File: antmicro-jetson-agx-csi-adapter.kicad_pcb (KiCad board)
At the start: 4 copper layers, 73.6 x 41 mm, 102 parts, among them IC1 MAX1708EEE+, J1 QTH-060-03-L-D-A, J2 WE_68715014522_ONE-SIDE, J3 WE_68715014022, J4 SM04B-SRSS-TB-LF-SN, J5 SM06B-SRSS-TB(LF)(SN), J6 SM09B-SRSS-TB(LF)(SN), Q1 BSS138AKA, U1 PCA9547BS,118, U2 NTS0102DP

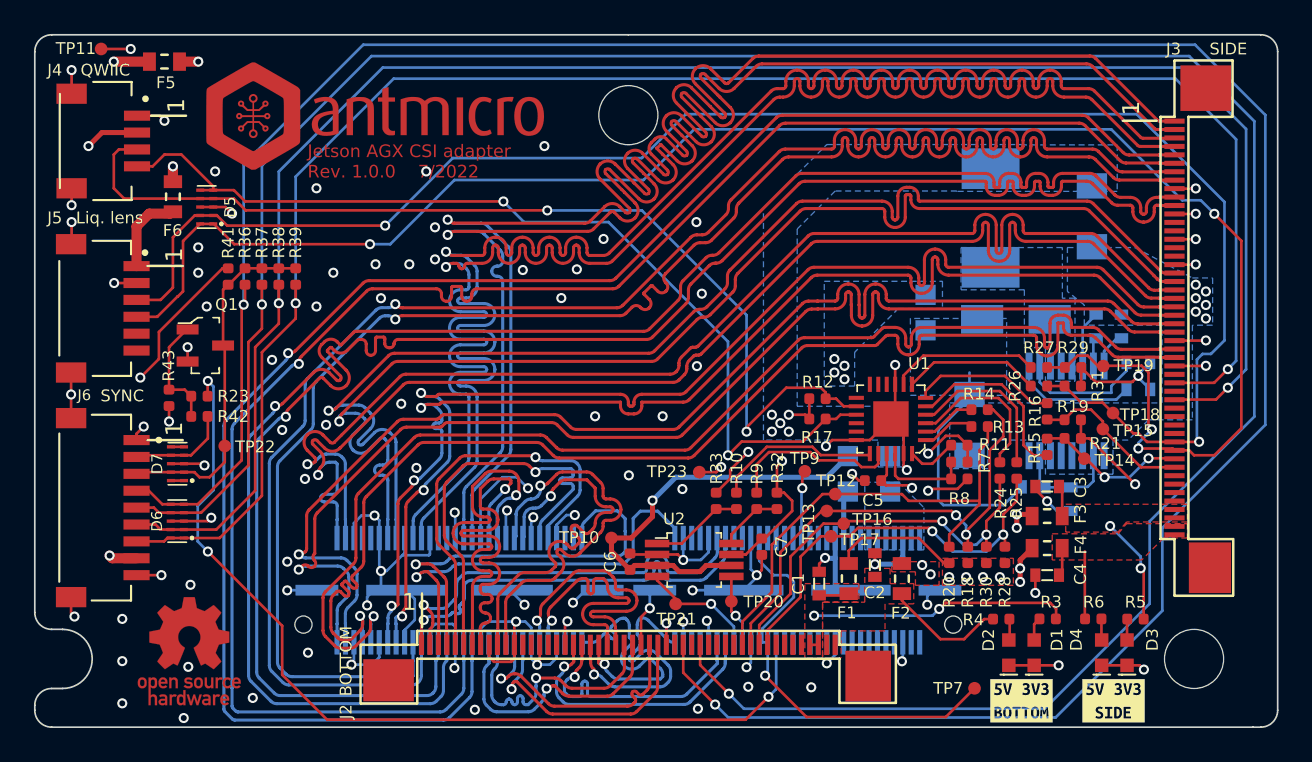
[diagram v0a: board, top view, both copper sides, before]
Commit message: [#60956] WiP Update symbols references
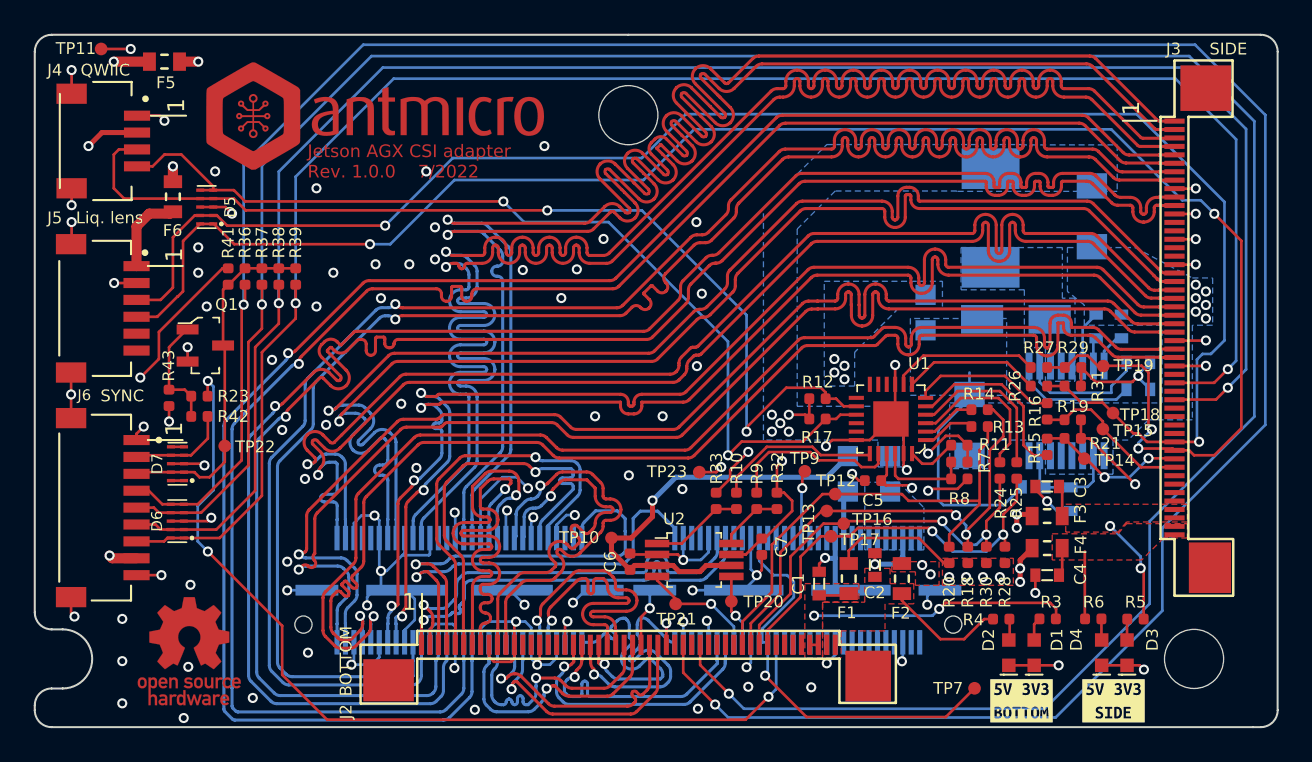
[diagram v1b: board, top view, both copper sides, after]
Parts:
- C1, C10, C11, C2, C3, C4, C9: footprint antmicro-jetson-agx-csi-adapter-footprints:0603-cap -> antmicro-footprints:C_0603_1608Metric
- C12, C8: footprint antmicro-jetson-agx-csi-adapter-footprints:1206-cap -> antmicro-footprints:C_1206_3216Metric
- C5, C6, C7: footprint antmicro-jetson-agx-csi-adapter-footprints:0402-cap -> antmicro-footprints:C_0402_1005Metric
- D1, D2, D3, D4: footprint antmicro-jetson-agx-csi-adapter-footprints:LED_0603 -> antmicro-footprints:LED_0603_1608Metric_G
- D5, D6, D7: footprint antmicro-jetson-agx-csi-adapter-footprints:PUSB3F96X -> antmicro-footprints:Nexperia_DFN-10_2.5x1mm_P0.5mm
- F1, F2, F3, F4, F5, F6: footprint antmicro-jetson-agx-csi-adapter-footprints:0603-Fuse-Littelfuse-0467 -> antmicro-footprints:F_0603_1608Metric
- J1: footprint antmicro-jetson-agx-csi-adapter-footprints:SAMTEC_QTH-060-03-X-D-A -> antmicro-footprints:Conn_Plug_Samtec_QTH_2x60_QTH-060-03-L-D-A
- J5: footprint antmicro-jetson-agx-csi-adapter-footprints:JST_SM06B-SRSS-TB(LF)(SN) -> antmicro-footprints:Conn_JST_GH_1x6_SM06B-GHS-TB-LF-SN
- J6: footprint antmicro-jetson-agx-csi-adapter-footprints:JST_SM09B-SRSS-TB(LF)(SN) -> antmicro-footprints:Conn_JST_SH_1x9_SM09B-SRSS-TB-LF-SN
- L1: footprint antmicro-jetson-agx-csi-adapter-footprints:IHLP2525CZER -> antmicro-footprints:L_2525_6363Metric
- Q1: footprint antmicro-jetson-agx-csi-adapter-footprints:SOT-23-3 -> antmicro-footprints:SOT-23-3
- R1, R2, R22: footprint antmicro-jetson-agx-csi-adapter-footprints:0805-res -> antmicro-footprints:R_0805_2012Metric
- R10, R11, R12, R13, R14, R15, R16, R17, R18, R19, R20, R21, R23, R24, R25, R26, R27, R28, R29, R3, R30, R31, R32, R33, R36, R37, R38, R39, R4, R41, R42, R43, R5, R6, R7, R8, R9: footprint antmicro-jetson-agx-csi-adapter-footprints:0402-res -> antmicro-footprints:R_0402_1005Metric
- R34, R35, R40: footprint antmicro-jetson-agx-csi-adapter-footprints:0603-res -> antmicro-footprints:R_0603_1608Metric
- U1: footprint antmicro-jetson-agx-csi-adapter-footprints:HVQFN24 -> antmicro-footprints:VQFN-24-1EP_3.8x3.8x1.0mm_P0.5mm
- U2: footprint antmicro-jetson-agx-csi-adapter-footprints:TSSOP-8_W3mm -> antmicro-footprints:TSSOP-8_3x3mm_P0.65mm
